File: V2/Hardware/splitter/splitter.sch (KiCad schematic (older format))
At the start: 21 parts, among them J0 Rpi_40Pin_F, J1 Control_seg:1, J2 Control_seg:2, J3 Control_seg:3, J4 Molex_PSU_F, J5 Siren, J6 USB_A_F, K0 RELRAS0515, Q1 BD139-16

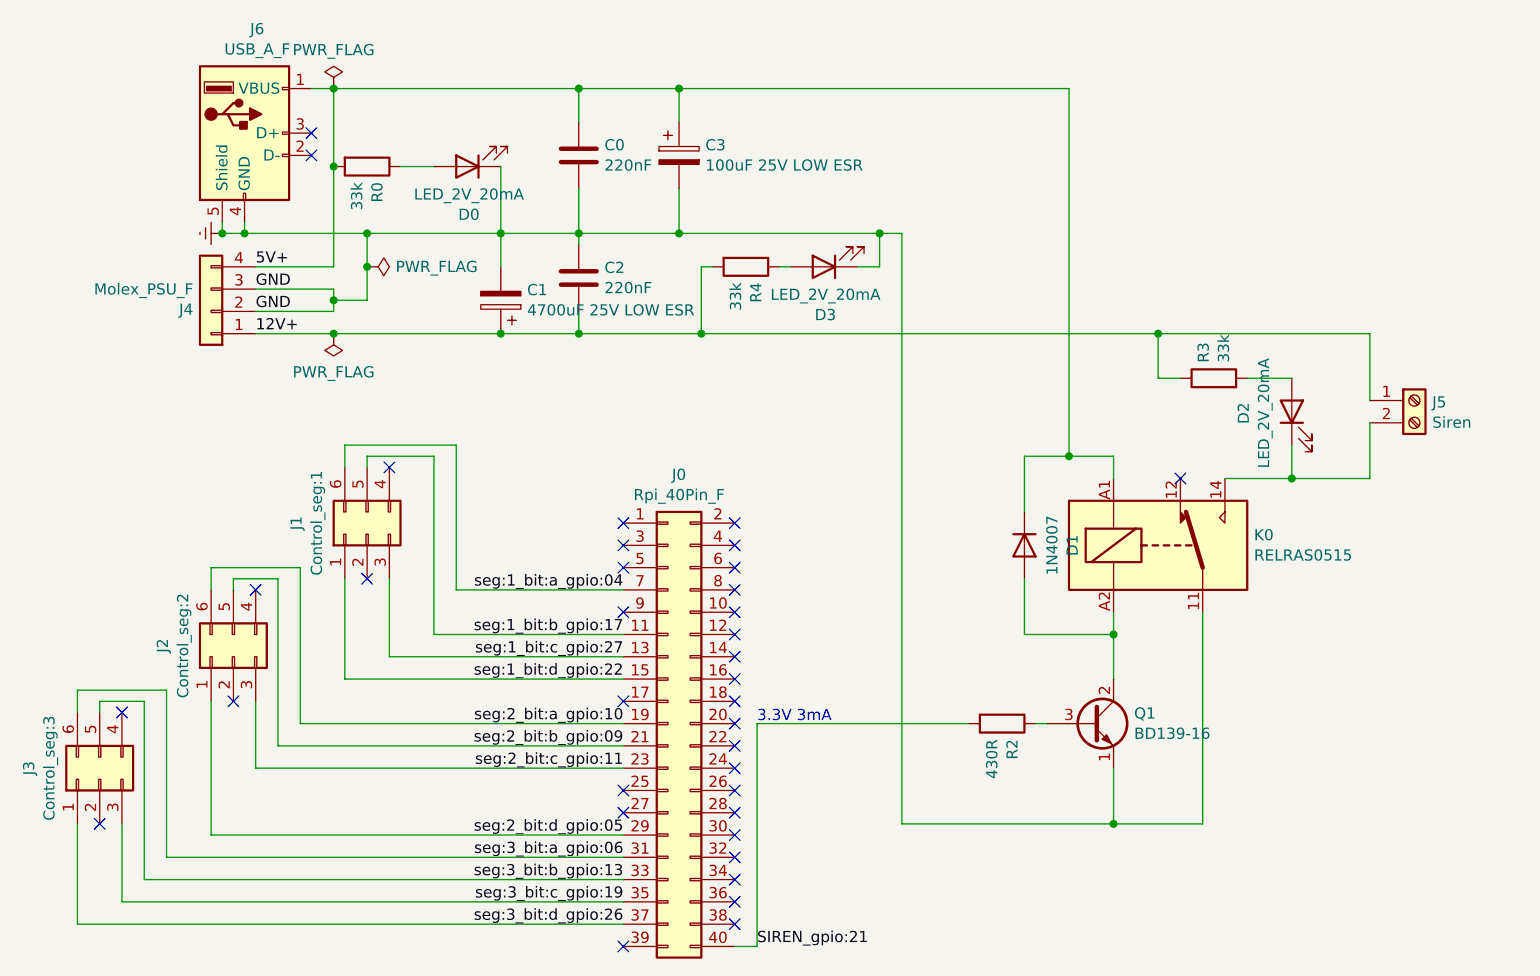
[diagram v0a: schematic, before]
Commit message: Update splitter
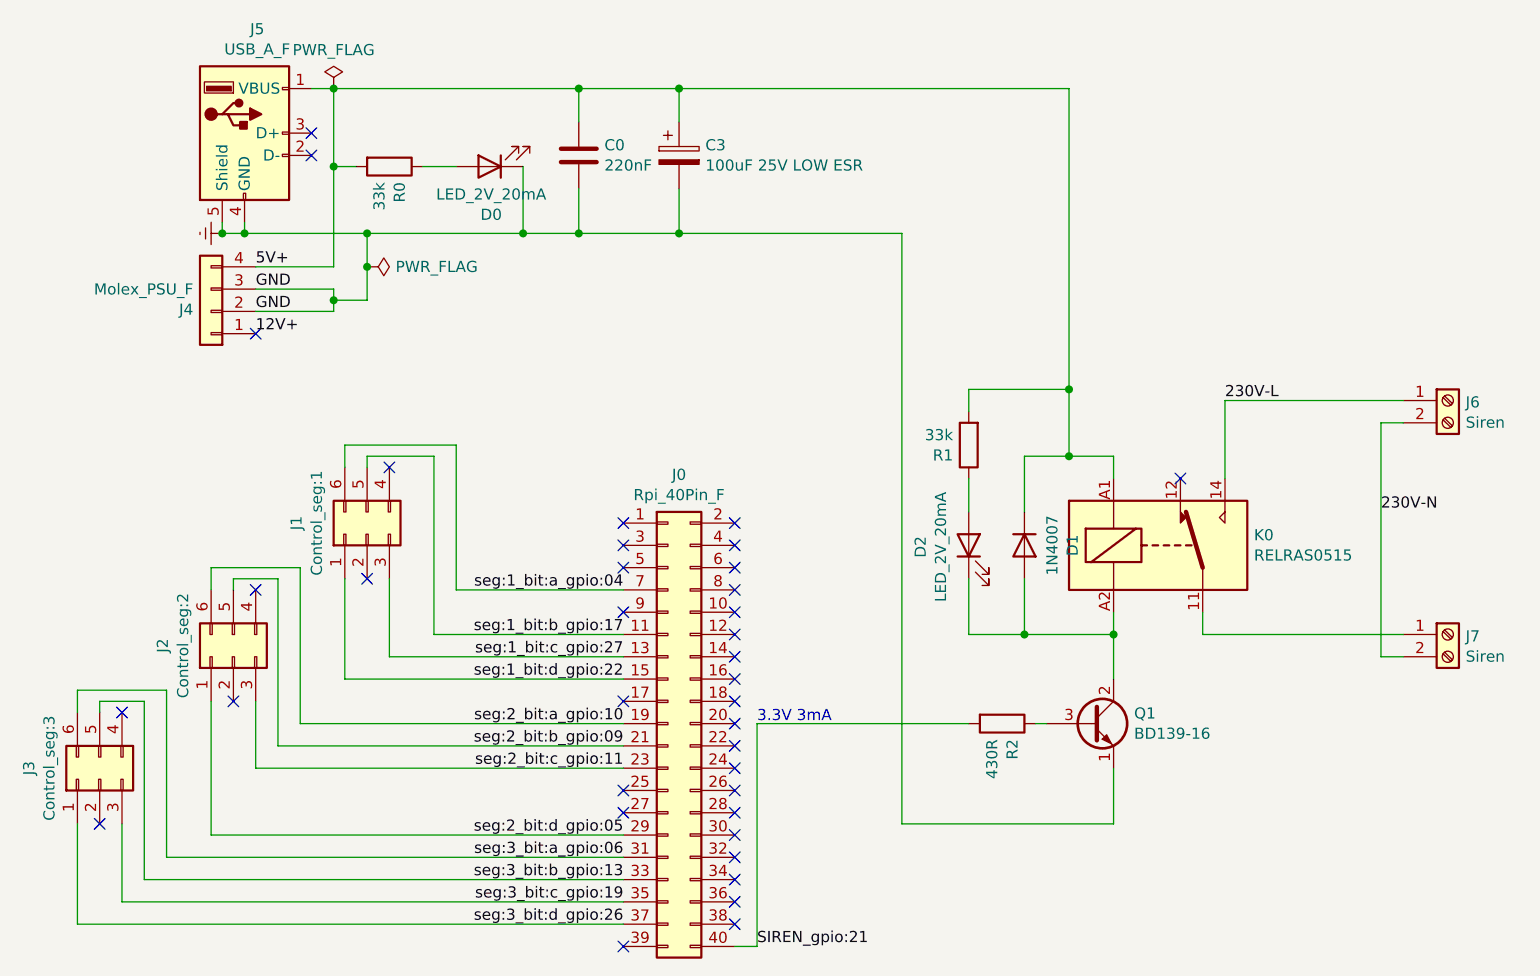
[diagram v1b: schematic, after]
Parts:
- removed C1: 4700uF 25V LOW ESR, Capacitor_THT:CP_Radial_D18.0mm_P7.50mm, symbol Device:CP
- removed C2: 220nF, Capacitor_THT:C_Disc_D4.3mm_W1.9mm_P5.00mm, symbol Device:C
- removed D3: LED_2V_20mA, LED_THT:LED_D5.0mm, symbol Device:LED
- removed R3, R4: 33k, Resistor_THT:R_Axial_DIN0207_L6.3mm_D2.5mm_P10.16mm_Horizontal, symbol Device:R
- added J7: Siren, TerminalBlock_RND:TerminalBlock_RND_205-00067_1x02_P7.50mm_Horizontal, symbol Connector:Screw_Terminal_01x02
- added R1: 33k, Resistor_THT:R_Axial_DIN0207_L6.3mm_D2.5mm_P10.16mm_Horizontal, symbol Device:R
- J6: renamed from J5; footprint TerminalBlock:TerminalBlock_bornier-2_P5.08mm -> TerminalBlock_RND:TerminalBlock_RND_205-00067_1x02_P7.50mm_Horizontal
- renumbered J6 to J5
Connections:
- net 12V+: no longer J6.1 (Pin_1)
- net 5V+: now also R1.2
- net Earth: no longer K0.11
- net at D1.2 (A), K0.A2, Q1.2 (C): now also D2.1 (K)
- net at D2.2 (A): now also R1.1
- new net: J7.1 (Pin_1), K0.11
- new net 230V-L: J6.1 (Pin_1), K0.14
- new net 230V-N: J6.2 (Pin_2), J7.2 (Pin_2)
- no-connect marks 36 -> 37
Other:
- moved on the sheet: D0, J6, R0
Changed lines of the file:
@@
 $EndComp
 $Comp
-L splitter-rescue:USB_A-Connector J6
+L splitter-rescue:USB_A-Connector J5
 U 1 1 5EBB092E
 P 3900 1950
-F 0 "J6" H 3957 2417 50  0000 C CNN
+F 0 "J5" H 3957 2417 50  0000 C CNN
 F 1 "USB_A_F" H 3957 2326 50  0000 C CNN
 F 2 "Connector_USB:USB_A_Stewart_SS-52100-001_Horizontal" H 4050 1900 50  0001 C CNN
@@
 $EndComp
 $Comp
-L Connector:Screw_Terminal_01x02 J5
+L Connector:Screw_Terminal_01x02 J6
 U 1 1 5EBB14C8
-P 9150 3150
-F 0 "J5" H 9230 3142 50  0000 L CNN
-F 1 "Siren" H 9230 3051 50  0000 L CNN
-F 2 "TerminalBlock:TerminalBlock_bornier-2_P5.08mm" H 9150 3150 50  0001 C CNN
-F 3 "~" H 9150 3150 50  0001 C CNN
-	1    9150 3150
+P 9300 3150
+F 0 "J6" H 9380 3142 50  0000 L CNN
+F 1 "Siren" H 9380 3051 50  0000 L CNN
+F 2 "TerminalBlock_RND:TerminalBlock_RND_205-00067_1x02_P7.50mm_Horizontal" H 9300 3150 50  0001 C CNN
+F 3 "~" H 9300 3150 50  0001 C CNN
+	1    9300 3150
 	1    0    0    -1
 $EndComp
@@
 L Device:R R0
 U 1 1 5EC190C2
-P 4450 2100
-F 0 "R0" H 4520 2146 50  0000 L CNN
-F 1 "33k" H 4520 2055 50  0000 L CNN
-F 2 "Resistor_THT:R_Axial_DIN0207_L6.3mm_D2.5mm_P10.16mm_Horizontal" V 4380 2100 50  0001 C CNN
-F 3 "~" H 4450 2100 50  0001 C CNN
-	1    4450 2100
+P 4550 2100
+F 0 "R0" H 4620 2146 50  0000 L CNN
+F 1 "33k" H 4620 2055 50  0000 L CNN
+F 2 "Resistor_THT:R_Axial_DIN0207_L6.3mm_D2.5mm_P10.16mm_Horizontal" V 4480 2100 50  0001 C CNN
+F 3 "~" H 4550 2100 50  0001 C CNN
+	1    4550 2100
 	0    1    1    0
 $EndComp
@@
 L Device:LED D0
 U 1 1 5EC196E4
-P 4900 2100
-F 0 "D0" H 4893 2316 50  0000 C CNN
-F 1 "LED_2V_20mA" H 4893 2225 50  0000 C CNN
-F 2 "LED_THT:LED_D5.0mm" H 4900 2100 50  0001 C CNN
-F 3 "~" H 4900 2100 50  0001 C CNN
-	1    4900 2100
+P 5000 2100
+F 0 "D0" H 4993 2316 50  0000 C CNN
+F 1 "LED_2V_20mA" H 4993 2225 50  0000 C CNN
+F 2 "LED_THT:LED_D5.0mm" H 5000 2100 50  0001 C CNN
+F 3 "~" H 5000 2100 50  0001 C CNN
+	1    5000 2100
 	-1   0    0    1
 $EndComp
@@
 	4300 2750 3950 2750
 Wire Wire Line
-	3950 2850 4300 2850
-Wire Wire Line
 	3950 2550 4300 2550
-Wire Wire Line
-	4300 2550 4300 2100
 Wire Wire Line
 	4300 1750 4200 1750
@@
 $EndComp
 Connection ~ 3800 2400
-$Comp
-L power:PWR_FLAG #FLG0102
-U 1 1 5EC7A631
-P 4300 2850
-F 0 "#FLG0102" H 4300 2925 50  0001 C CNN
-F 1 "PWR_FLAG" H 4300 3023 50  0000 C CNN
-F 2 "" H 4300 2850 50  0001 C CNN
-F 3 "~" H 4300 2850 50  0001 C CNN
-	1    4300 2850
-	-1   0    0    1
-$EndComp
-Connection ~ 4300 2850
 NoConn ~ 4200 1950
 NoConn ~ 4200 2050
@@
 	4450 2550 4450 2400
 Wire Wire Line
-	4450 2400 5050 2400
+	4450 2400 5150 2400
 Connection ~ 4450 2400
-Connection ~ 4300 2100
-Wire Wire Line
-	4300 2100 4300 1750
-Wire Wire Line
-	4600 2100 4750 2100
-Wire Wire Line
-	5050 2100 5050 2400
-Connection ~ 5050 2400
+Wire Wire Line
+	5150 2100 5150 2400
+Connection ~ 5150 2400
 $Comp
 L power:PWR_FLAG #FLG0103
@@
 	7450 4600 7500 4600
 Wire Wire Line
-	4300 2850 5050 2850
-Wire Wire Line
 	6850 5050 7800 5050
 Wire Wire Line
@@
 Wire Wire Line
 	7800 3400 7800 3500
-Wire Wire Line
-	8200 4100 8200 5050
-Wire Wire Line
-	8200 5050 7800 5050
-Connection ~ 7800 5050
 NoConn ~ 8100 3500
 NoConn ~ 6100 4100
-$Comp
-L Device:LED D2
-U 1 1 5EDC36BC
-P 8600 3200
-F 0 "D2" H 8593 3416 50  0000 C CNN
-F 1 "LED_2V_20mA" H 8593 3325 50  0000 C CNN
-F 2 "LED_THT:LED_D5.0mm" H 8600 3200 50  0001 C CNN
-F 3 "~" H 8600 3200 50  0001 C CNN
-	1    8600 3200
-	0    -1   -1   0
-$EndComp
-$Comp
-L Device:R R3
-U 1 1 5EDC8D2F
-P 8250 3050
-F 0 "R3" H 8320 3096 50  0000 L CNN
-F 1 "33k" H 8320 3005 50  0000 L CNN
-F 2 "Resistor_THT:R_Axial_DIN0207_L6.3mm_D2.5mm_P10.16mm_Horizontal" V 8180 3050 50  0001 C CNN
-F 3 "~" H 8250 3050 50  0001 C CNN
-	1    8250 3050
-	0    -1   -1   0
-$EndComp
 NoConn ~ 6100 4200
 $Comp
@@
 Wire Wire Line
 	3450 5300 5600 5300
-$Comp
-L Device:R R4
-U 1 1 5FCA692B
-P 6150 2550
-F 0 "R4" H 6220 2596 50  0000 L CNN
-F 1 "33k" H 6220 2505 50  0000 L CNN
-F 2 "Resistor_THT:R_Axial_DIN0207_L6.3mm_D2.5mm_P10.16mm_Horizontal" V 6080 2550 50  0001 C CNN
-F 3 "~" H 6150 2550 50  0001 C CNN
-	1    6150 2550
-	0    1    1    0
-$EndComp
-$Comp
-L Device:LED D3
-U 1 1 5FCABBDF
-P 6500 2550
-F 0 "D3" H 6493 2766 50  0000 C CNN
-F 1 "LED_2V_20mA" H 6493 2675 50  0000 C CNN
-F 2 "LED_THT:LED_D5.0mm" H 6500 2550 50  0001 C CNN
-F 3 "~" H 6500 2550 50  0001 C CNN
-	1    6500 2550
-	-1   0    0    1
-$EndComp
-Wire Wire Line
-	5950 2850 5950 2550
-Wire Wire Line
-	5950 2550 6000 2550
-Connection ~ 5950 2850
-Wire Wire Line
-	6300 2550 6350 2550
-Wire Wire Line
-	6650 2550 6750 2550
-Wire Wire Line
-	6750 2550 6750 2400
-Connection ~ 6750 2400
-Wire Wire Line
-	6750 2400 6850 2400
 Wire Wire Line
 	4850 4000 5600 4000
@@
 	6200 4600 7150 4600
 Wire Wire Line
-	7600 3400 7600 1750
+	7600 3400 7600 3100
 Wire Wire Line
 	4300 1750 5400 1750
@@
 Wire Wire Line
 	7600 3400 7400 3400
-Wire Wire Line
-	8950 2850 8950 3150
-Wire Wire Line
-	8300 3500 8600 3500
-Wire Wire Line
-	8950 3500 8950 3250
-Wire Wire Line
-	8600 3050 8400 3050
-Wire Wire Line
-	8100 3050 8000 3050
-Wire Wire Line
-	8000 3050 8000 2850
-Connection ~ 8000 2850
-Wire Wire Line
-	8000 2850 8950 2850
-Wire Wire Line
-	8600 3350 8600 3500
-Connection ~ 8600 3500
-Wire Wire Line
-	8600 3500 8950 3500
 Text Notes 6200 4600 0    50   ~ 0
 3.3V 3mA
-$Comp
-L Device:CP C1
-U 1 1 5FDD03EF
-P 5050 2700
-F 0 "C1" H 4932 2654 50  0000 R CNN
-F 1 "4700uF 25V LOW ESR" H 4932 2745 50  0000 R CNN
-F 2 "Capacitor_THT:CP_Radial_D18.0mm_P7.50mm" H 5088 2550 50  0001 C CNN
-F 3 "~" H 5050 2700 50  0001 C CNN
-	1    5050 2700
-	-1   0    0    1
-$EndComp
-Wire Wire Line
-	5050 2550 5050 2400
-Wire Wire Line
-	5050 2400 5400 2400
-Connection ~ 5050 2850
-Wire Wire Line
-	5050 2850 5400 2850
-$Comp
-L Device:C C2
-U 1 1 5FE2424F
-P 5400 2600
-F 0 "C2" H 5515 2646 50  0000 L CNN
-F 1 "220nF" H 5515 2555 50  0000 L CNN
-F 2 "Capacitor_THT:C_Disc_D4.3mm_W1.9mm_P5.00mm" H 5438 2450 50  0001 C CNN
-F 3 "~" H 5400 2600 50  0001 C CNN
-	1    5400 2600
-	1    0    0    -1
-$EndComp
-Wire Wire Line
-	5400 2450 5400 2400
+Wire Wire Line
+	5150 2400 5400 2400
 Connection ~ 5400 2400
 Wire Wire Line
 	5400 2400 5850 2400
-Wire Wire Line
-	5400 2750 5400 2850
-Connection ~ 5400 2850
-Wire Wire Line
-	5400 2850 5950 2850
 $Comp
 L Device:C C0
@@
 Connection ~ 5850 2400
 Wire Wire Line
-	5850 2400 6750 2400
-Wire Wire Line
-	5950 2850 8000 2850
-Wire Wire Line
 	6850 2400 6850 5050
+Wire Wire Line
+	5850 2400 6850 2400
+NoConn ~ 3950 2850
+Wire Wire Line
+	4300 1750 4300 2100
+Wire Wire Line
+	4700 2100 4850 2100
+Wire Wire Line
+	4400 2100 4300 2100
+Connection ~ 4300 2100
+Wire Wire Line
+	4300 2100 4300 2550
+$Comp
+L Connector:Screw_Terminal_01x02 J7
+U 1 1 60876BBF
+P 9300 4200
+F 0 "J7" H 9380 4192 50  0000 L CNN
+F 1 "Siren" H 9380 4101 50  0000 L CNN
+F 2 "TerminalBlock_RND:TerminalBlock_RND_205-00067_1x02_P7.50mm_Horizontal" H 9300 4200 50  0001 C CNN
+F 3 "~" H 9300 4200 50  0001 C CNN
+	1    9300 4200
+	1    0    0    -1
+$EndComp
+Text Label 9000 3650 0    50   ~ 0
+230V-N
+Text Label 8300 3150 0    50   ~ 0
+230V-L
+$Comp
+L Device:LED D2
+U 1 1 60899463
+P 7150 3800
+F 0 "D2" H 7143 4016 50  0000 C CNN
+F 1 "LED_2V_20mA" H 7143 3925 50  0000 C CNN
+F 2 "LED_THT:LED_D5.0mm" H 7150 3800 50  0001 C CNN
+F 3 "~" H 7150 3800 50  0001 C CNN
+	1    7150 3800
+	0    -1   -1   0
+$EndComp
+$Comp
+L Device:R R1
+U 1 1 6089AC25
+P 7150 3350
+F 0 "R1" H 7220 3396 50  0000 L CNN
+F 1 "33k" H 7220 3305 50  0000 L CNN
+F 2 "Resistor_THT:R_Axial_DIN0207_L6.3mm_D2.5mm_P10.16mm_Horizontal" V 7080 3350 50  0001 C CNN
+F 3 "~" H 7150 3350 50  0001 C CNN
+	1    7150 3350
+	-1   0    0    1
+$EndComp
+Wire Wire Line
+	7150 3650 7150 3500
+Wire Wire Line
+	7150 3200 7150 3100
+Wire Wire Line
+	7150 3100 7600 3100
+Connection ~ 7600 3100
+Wire Wire Line
+	7600 3100 7600 1750
+Wire Wire Line
+	7150 3950 7150 4200
+Wire Wire Line
+	7150 4200 7400 4200
+Connection ~ 7400 4200
+Wire Wire Line
+	8200 4100 8200 4200
+Wire Wire Line
+	8200 4200 9100 4200
+Wire Wire Line
+	8300 3500 8300 3150
+Wire Wire Line
+	8300 3150 9100 3150
+Wire Wire Line
+	9100 3250 9000 3250
+Wire Wire Line
+	9000 3250 9000 4300
+Wire Wire Line
+	9000 4300 9100 4300
 $EndSCHEMATC
